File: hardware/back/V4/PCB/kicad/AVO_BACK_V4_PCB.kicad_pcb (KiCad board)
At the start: 4 copper layers, 46.7 x 47.4 mm, 105 parts, among them J1 USB-C 16P, J2 BATERÍA 1S, J3 microSD DM3AT, J4 URTK1.2 (8 hilos), Q1 AO3401A, Q2 AO3401A, Q3 AO3401A, Q4 AO3401A, U1 BQ51013BRHLR, U2 BQ24072RGTR, U3 TLV75733PDBVR, U4 ESP32-S3-MINI-1U-N8, U6 USBLC6-2SC6, U7 RT9080-33GJ5, U8 DRV5032FADBZR

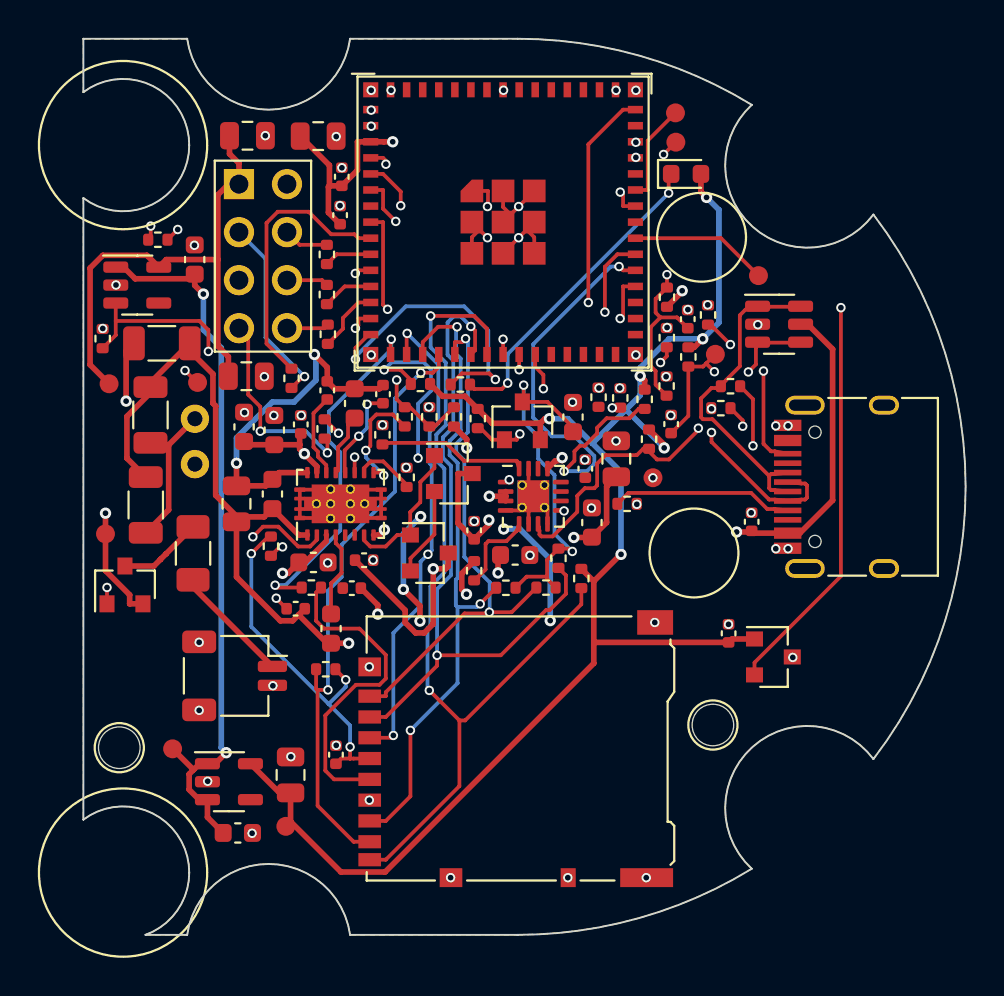
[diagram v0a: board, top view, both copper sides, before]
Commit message: PCB espalda V4: resultados de KiCad 9 de 207f2bd (puerta: false) [skip ci]
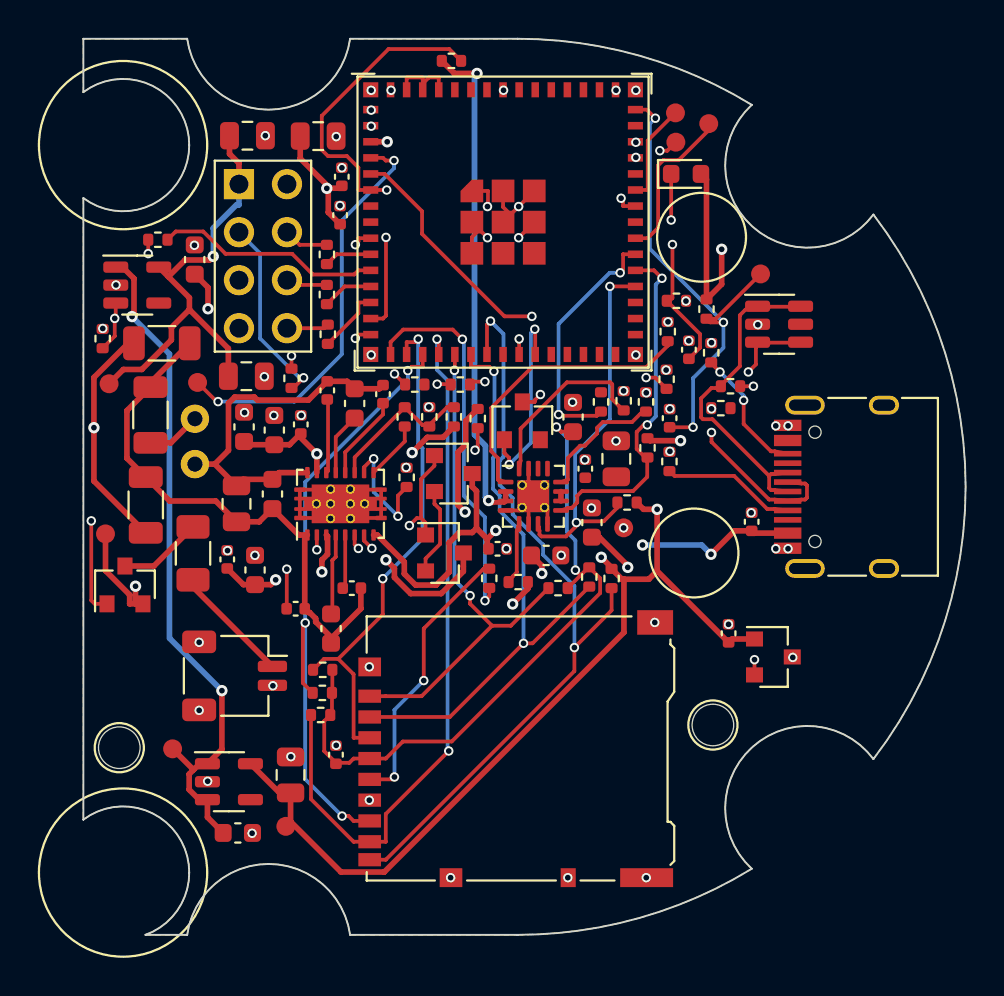
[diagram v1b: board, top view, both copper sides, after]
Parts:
- moved R32 16.9 mm to (85.2, 77.5), turned to 0 degrees
- moved R6 12.9 mm to (94.3, 95.5)
- moved R42 11.2 mm to (78.3, 110.9)
- moved R4 9.60 mm to (93.1, 95.5), turned to 90 degrees
- moved R46 9.42 mm to (87.2, 104.8), turned to 90 degrees
- moved TP10 8.46 mm to (98.8, 80.8)
- moved C16 7.24 mm to (73.3, 103.8), turned to 90 degrees
- moved R41 7.09 mm to (78.4, 109.7), turned to 0 degrees
- moved R55 5.32 mm to (83.2, 94.6), turned to 0 degrees
- moved TP1 4.88 mm to (101.5, 88.7)
- moved R33 4.54 mm to (97.1, 90.2), turned to 0 degrees
- moved RT2 4.32 mm to (96.6, 91.8)
- moved R9 3.55 mm to (94.5, 100.8), turned to 0 degrees
- moved R16 3.17 mm to (96.7, 98.7), turned to 90 degrees
- moved C15 3.12 mm to (74.8, 104.4), turned to 90 degrees
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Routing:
- net VIN5: track 60.1 -> 18.0 mm, vias 5 -> 3
- net VBAT: track 84.5 -> 59.5 mm, vias 7 -> 4
- net USB_DM: track 19.0 -> 0.00 mm, vias 2 -> 0
- net ZED_PPS: track 16.2 -> 0.00 mm, vias 2 -> 0
- net +3V3_SD: track 53.2 -> 38.9 mm, vias 5 -> 3
- net BAT_ADC: track 27.2 -> 40.9 mm
- net +3V3: track 112.9 -> 125.6 mm
- net VBUS: track 42.2 -> 32.1 mm
- net QI_AC1: track 38.8 -> 28.9 mm, vias 2 -> 0
- net LED: track 16.0 -> 6.97 mm
- net HALL: track 49.6 -> 41.6 mm
- net CHG_TS: track 7.67 -> 15.3 mm, vias 2 -> 0
- net SD_CMD: track 34.3 -> 27.1 mm, vias 4 -> 2
- net CHG_STAT: track 25.7 -> 18.6 mm, vias 3 -> 2
- net CHG_ILIM: track 0.00 -> 6.84 mm
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
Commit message: PCB espalda V4: resultados de KiCad 9 de 3f81b45 (puerta: true) [skip ci]
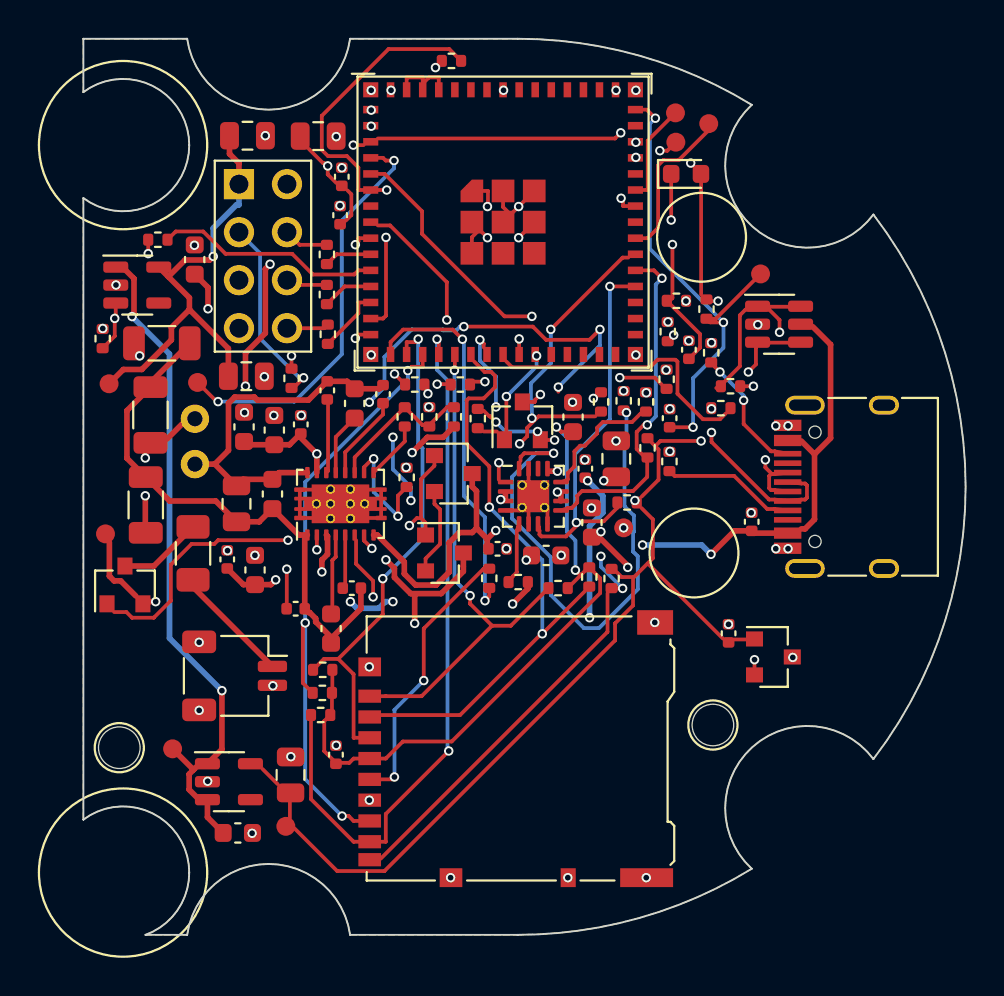
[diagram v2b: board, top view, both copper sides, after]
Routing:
- net +3V3: track 125.6 -> 99.1 mm, vias 7 -> 11
- net VIN5: track 18.0 -> 39.0 mm, vias 3 -> 7
- net CHG_TS: track 15.3 -> 36.2 mm, vias 0 -> 8
- net CHG_ISET: track 9.67 -> 27.7 mm, vias 0 -> 2
- net USB_DM: track 0.00 -> 14.3 mm
- net VBUS: track 32.1 -> 44.9 mm
- net QI_COIL1: track 20.6 -> 8.53 mm, vias 1 -> 3
- net ZED_PPS: track 0.00 -> 12.0 mm, vias 0 -> 2
- net SD_PWR_N: track 13.8 -> 5.36 mm, vias 3 -> 2
- net VSYS: track 71.2 -> 76.2 mm, vias 5 -> 8
- net SD_CD: track 41.3 -> 36.9 mm, vias 2 -> 4
- net BAT_G: track 38.9 -> 35.6 mm
- net VBAT: track 59.5 -> 61.9 mm, vias 4 -> 8
- net USB_DP_C: track 18.0 -> 20.4 mm, vias 0 -> 2
- net QI_CHG: track 28.8 -> 30.7 mm, vias 3 -> 4
